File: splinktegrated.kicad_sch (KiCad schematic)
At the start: 160 parts, among them J1 USB_C_Receptacle_USB2.0, J10 NA_Ribbon, J13 Conn_01x01_Socket, J14 Cirque, J15 Conn_01x01_Socket, J16 Conn_01x01_Socket, J17 Conn_01x01_Socket, J18 USB_C_Receptacle_USB2.0, J19 Conn_01x01_Socket, J20 Conn_01x01_Socket, J5 Conn_01x02, J7 NA_trackball, J8 NA_Ribbon, J9 NA_RGB, Q4 AO3401A, Q5 AO3401A, SW2 NA_SW_SPST, SW9001 NA_SW_SPST, U1 RP2040, U2 USBLC6-2P6, U3 XC6210B332MR-G, U4 USBLC6-2P6, U5 W25Q128JVS, U6 74LVC1T45, Y1 Crystal_GND24

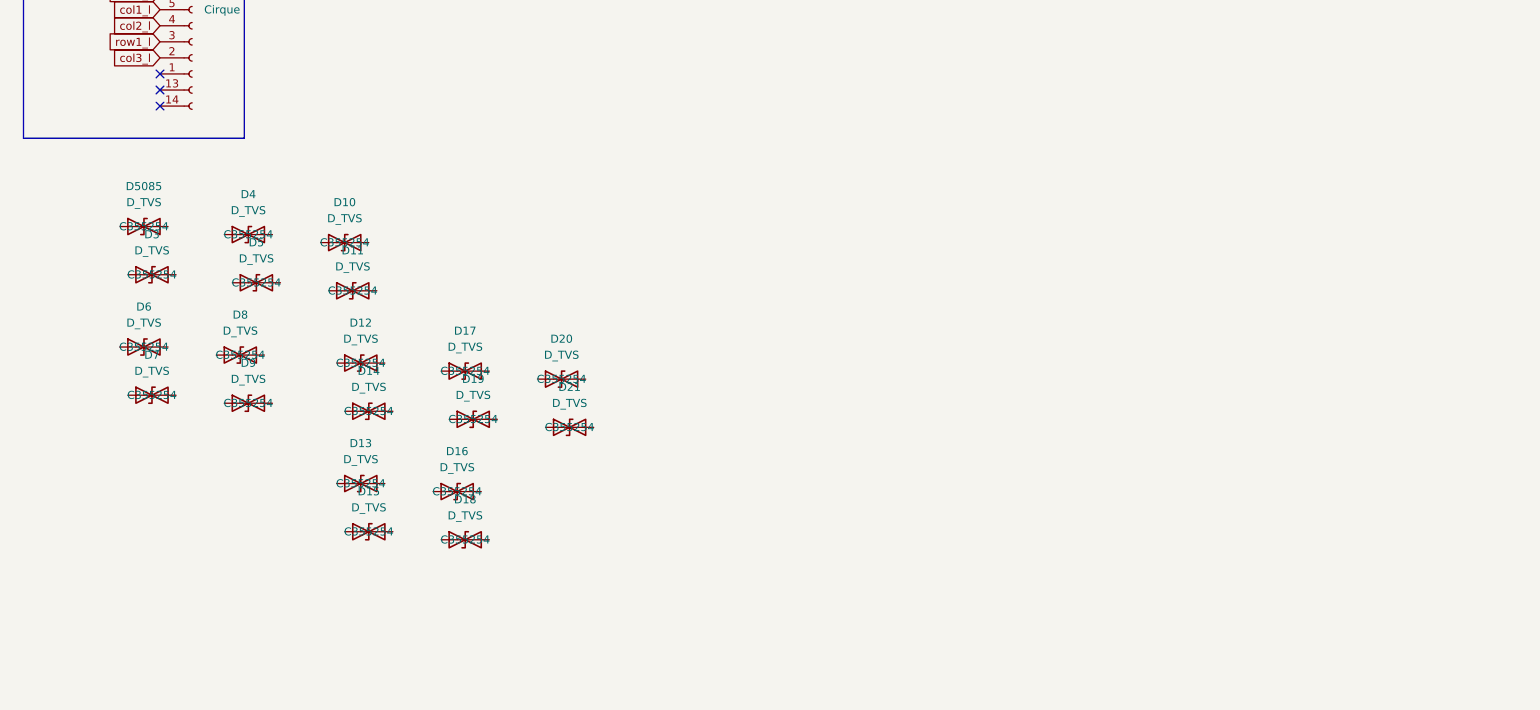
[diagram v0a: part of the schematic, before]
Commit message: routing
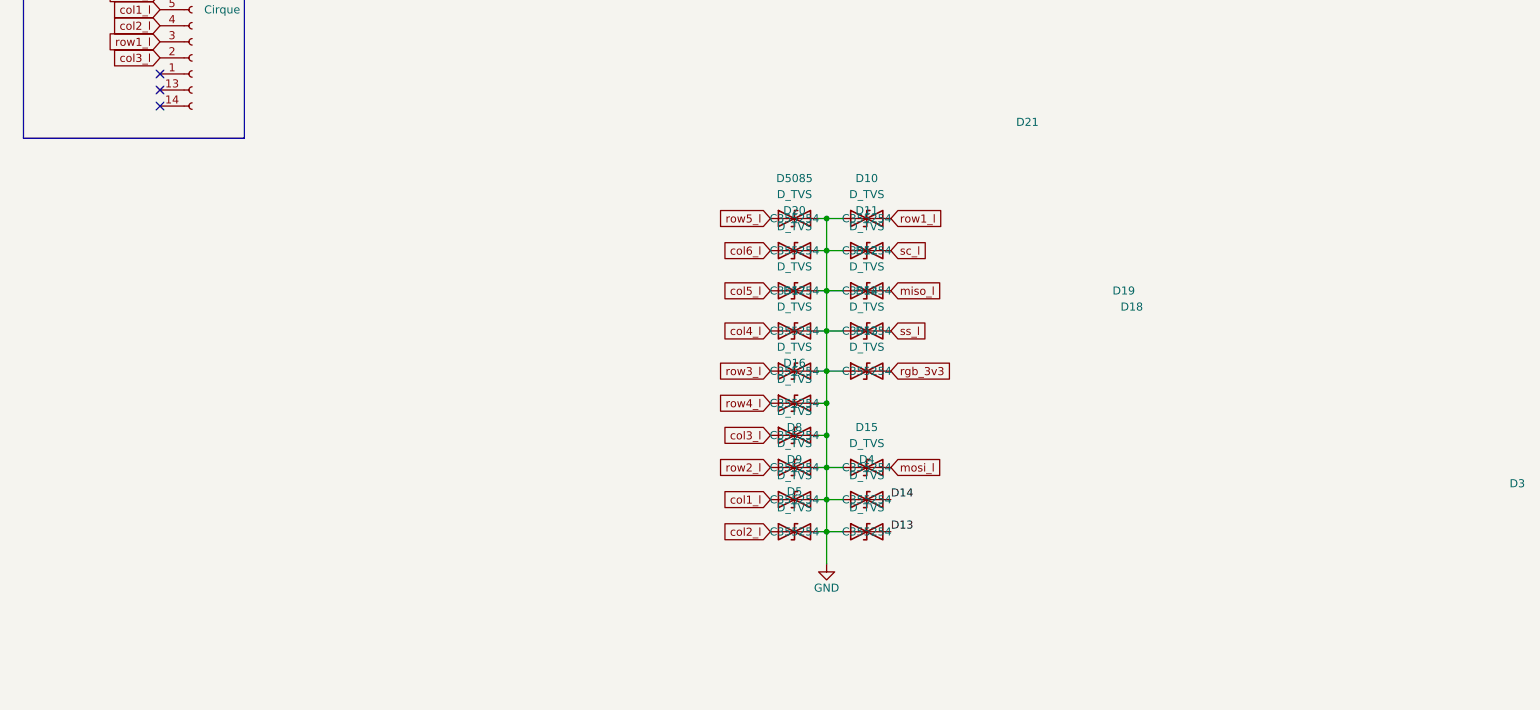
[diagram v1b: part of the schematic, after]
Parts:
- removed D6, D7: D_TVS, Diode_SMD:D_SOD-523, symbol Device:D_TVS
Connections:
- net D13: now also D3.2 (A2)
- net D14: now also D4.2 (A2)
- net GND: now also D10.1 (A1), D11.1 (A1), D12.1 (A1), D13.1 (A1), D14.1 (A1), D15.1 (A1), D16.2 (A2), D17.2 (A2), D18.2 (A2), D19.2 (A2), D20.2 (A2), D21.2 (A2), D3.1 (A1), D4.1 (A1), D5.2 (A2), D5085.2 (A2), D8.2 (A2), D9.2 (A2)
- net col1_l: now also D9.1 (A1)
- net col2_l: now also D5.1 (A1)
- net col3_l: now also D18.1 (A1)
- net col4_l: now also D17.1 (A1)
- net col5_l: now also D21.1 (A1)
- net col6_l: now also D20.1 (A1)
- net miso_l: now also D12.2 (A2)
- net mosi_l: now also D15.2 (A2)
- net rgb_3v3: now also D13.2 (A2)
- net row1_l: now also D10.2 (A2)
- net row2_l: now also D8.1 (A1)
- net row3_l: now also D19.1 (A1)
- net row4_l: now also D16.1 (A1)
- net row5_l: now also D5085.1 (A1)
- net sc_l: now also D11.2 (A2)
- net ss_l: now also D14.2 (A2)
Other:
- moved on the sheet: D10, D11, D12, D13, D14, D15, D16, D17, D18, D19, D20, D21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
